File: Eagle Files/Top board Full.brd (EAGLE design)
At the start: 21.8 x 20.3 mm, 19 parts

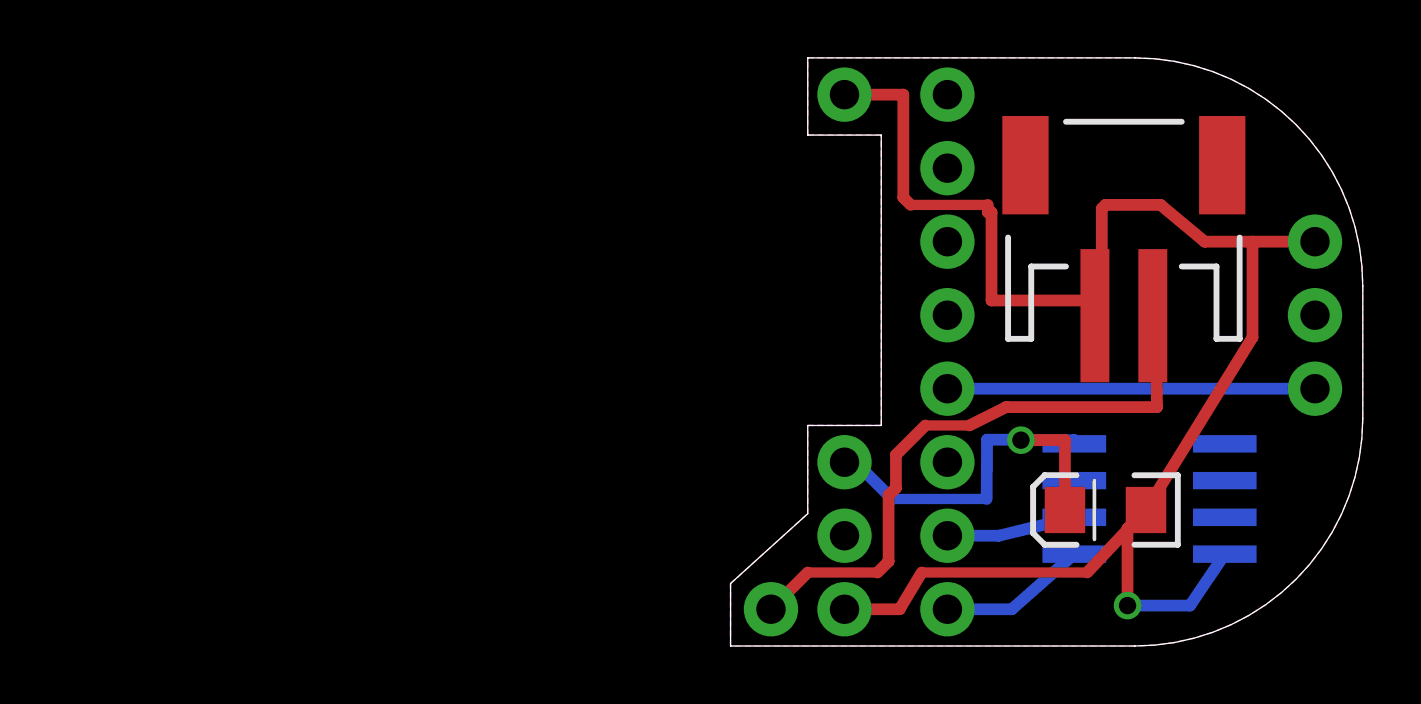
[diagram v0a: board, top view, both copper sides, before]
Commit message: Misc Changes
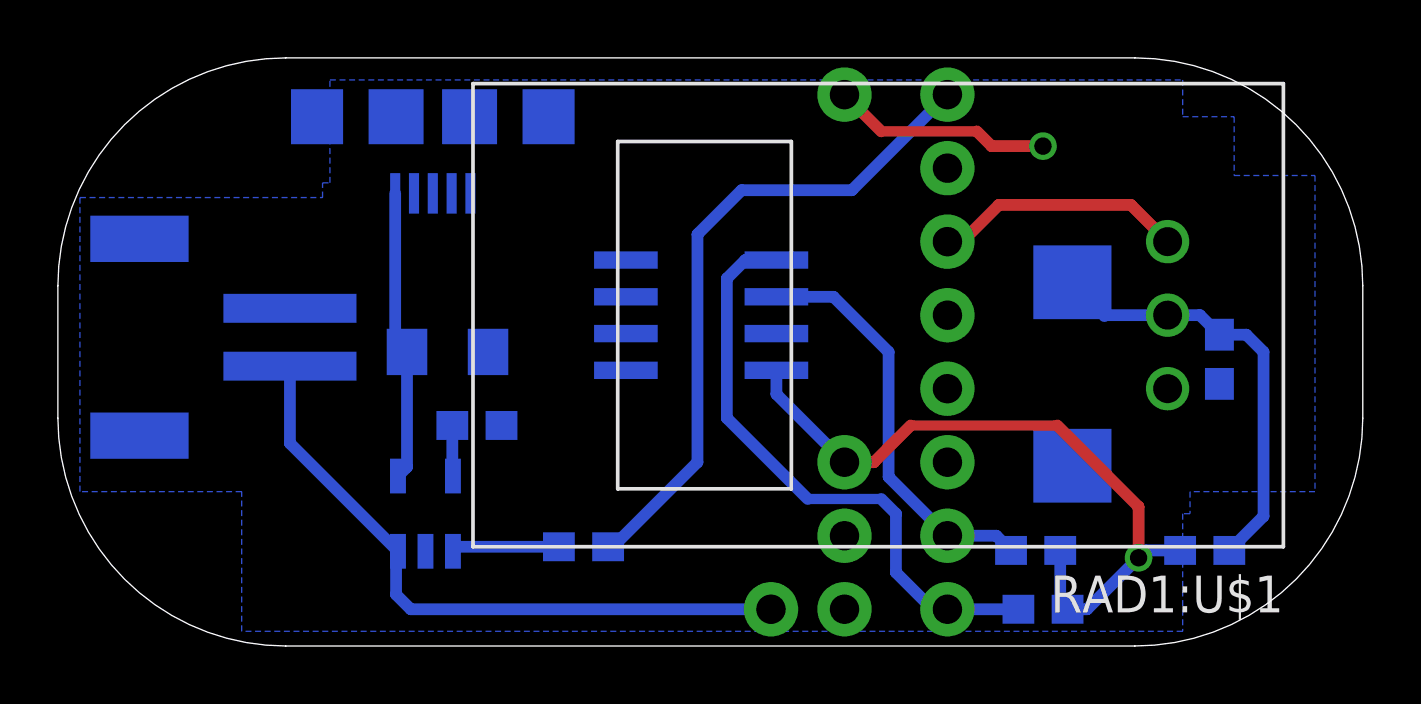
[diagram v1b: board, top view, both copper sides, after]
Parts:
- removed 4V, DATA, GND@1: PROTO_POINT, BLEduino Bean:1X01
- removed C1: 10uF, SparkFun-Capacitors:EIA3216
- removed J1: (no value), SparkFun-Connectors:JST-2-SMD
- added PWR1:C1: 10uF, SparkFun-Capacitors:EIA3216
- added PWR1:IC1: MCP73831/OT, adafruit:SOT23-5L
- added PWR1:J2: (no value), SparkFun-Connectors:JST-2-SMD
- added PWR1:JP1: USB-MICROB, SparkFun-Connectors:USB-MICROB
- added PWR1:R1: 470, SparkFun-Resistors:0603-RES
- added PWR1:R2: 2000, SparkFun-Resistors:0603-RES
- added R2, R3: 10K, SparkFun-Resistors:0603-RES
- added RAD1:C2: 100uF, SparkFun-Capacitors:EIA7343
- added RAD1:C3: 10pF, SparkFun-Capacitors:0603-CAP
- added RAD1:R1: 150, SparkFun-Resistors:0603-RES
- added RAD1:U$1: RD2007, radiationbean:RD2007
- moved FRAM 16.7 mm to (22.2, 11.4), turned to 90 degrees
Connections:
- removed net 4V: 4V.1
- removed net A0: FRAM.A0
- removed net A1: FRAM.A1
- removed net N$7: 0.1
- new net PWR1:N$1: PWR1:IC1.1, PWR1:R1.2
- new net PWR1:N$2: PWR1:IC1.5, PWR1:R2.2
- new net PWR1:VBUS: PWR1:C1.A, PWR1:IC1.4, PWR1:JP1.VBUS
- new net RAD1:V_SENS: RAD1:C2.A, RAD1:C3.1, RAD1:R1.2, RAD1:U$1.VCC
- net A2: now also 0.1; no longer FRAM.A2
- net CLK: now also PWR1:R1.1
- net DATA: no longer DATA.1
- net GND: now also PWR1:C1.C, PWR1:IC1.2, PWR1:J2.1, PWR1:JP1.GND, PWR1:JP1.MT1, PWR1:JP1.MT2, PWR1:R2.1, RAD1:C2.C, RAD1:C3.2, RAD1:U$1.GND; no longer C1.C, GND@1.1, J1.1
- net MOSI: now also RAD1:U$1.OUT
- net SCL: now also R3.2
- net SDA: now also R2.2
- net VBAT: now also PWR1:IC1.3, PWR1:J2.2; no longer J1.2
- net VCC: now also R2.1, R3.1, RAD1:R1.1; no longer C1.A
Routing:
- net GND: track 57.9 -> 7.59 mm
- net CLK: track 0.00 -> 22.8 mm
- net SDA: track 5.11 -> 20.8 mm
- net RAD1:V_SENS: track 0.00 -> 15.0 mm
- net DATA: track 12.7 -> 0.00 mm
- net PWR1:VBUS: track 0.00 -> 10.1 mm
- net VCC: track 14.6 -> 24.6 mm
- net SCL: track 4.46 -> 14.3 mm
- net MOSI: track 0.00 -> 8.66 mm
- net PWR1:N$1: track 0.00 -> 3.73 mm
- net PWR1:N$2: track 0.00 -> 1.76 mm
- net VBAT: track 21.3 -> 22.6 mm
- removed copper zone on layer 1, net GND
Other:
- board size 21.8 x 20.3 mm -> 45.1 x 20.3 mm
- board text added: "v0.1"
- board text removed: "Top Board"
- board text removed: "v0.2"
